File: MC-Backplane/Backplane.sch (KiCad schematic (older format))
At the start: 1 part

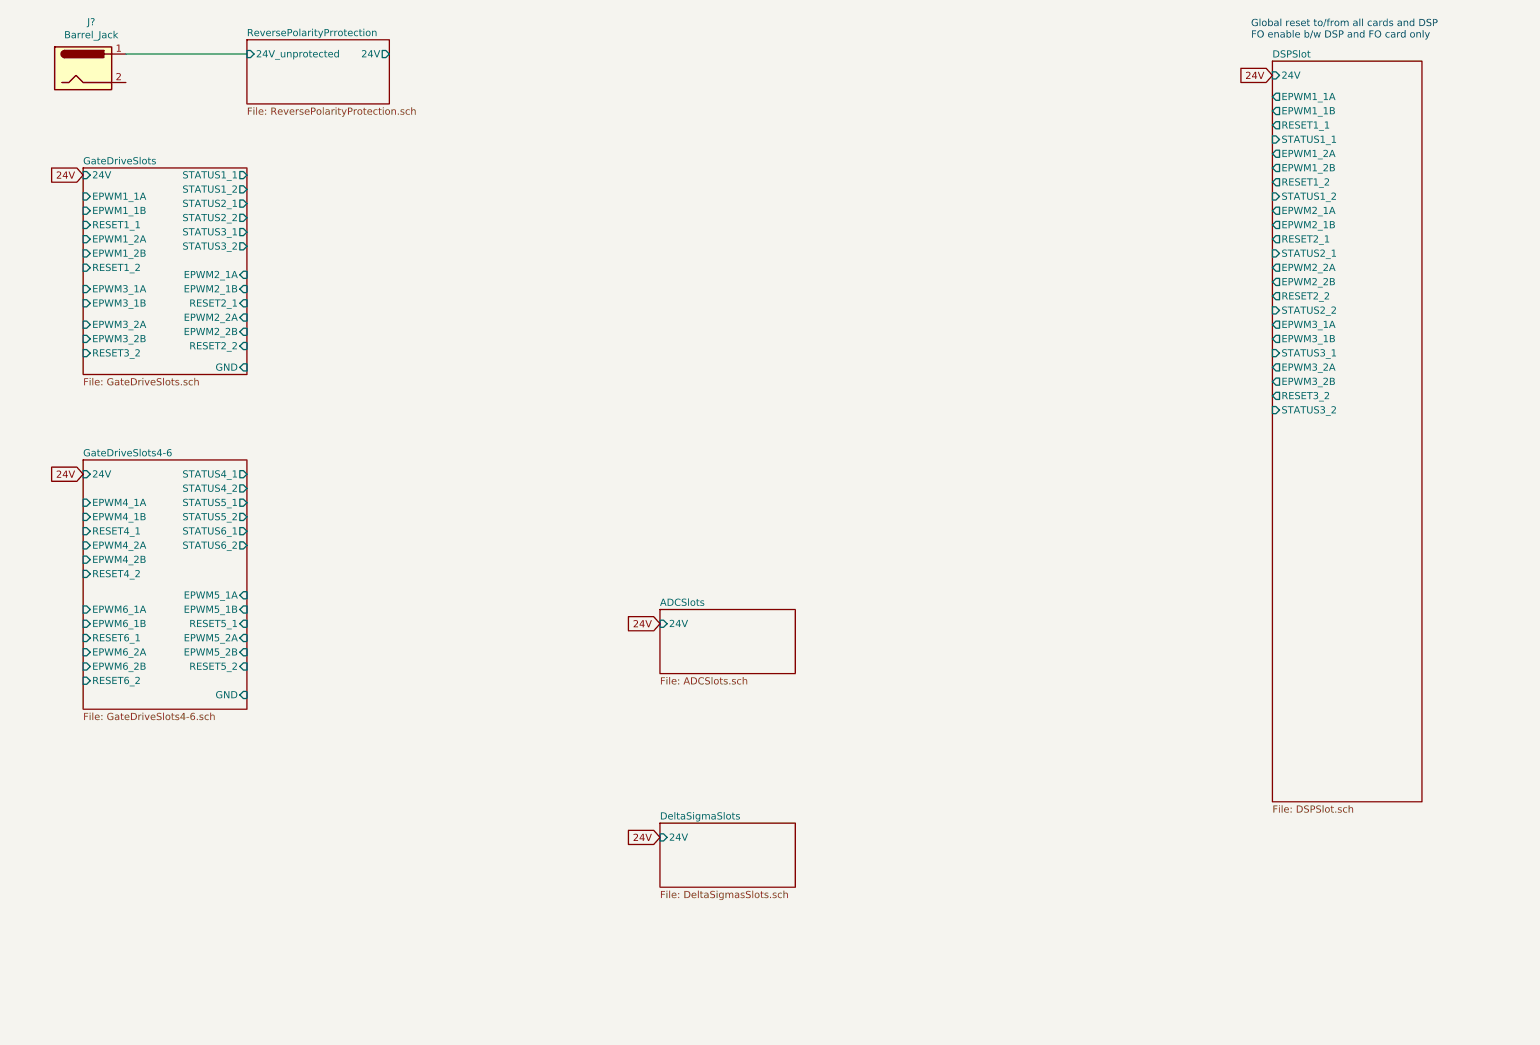
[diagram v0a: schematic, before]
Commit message: Add files via upload
updating net names and wires
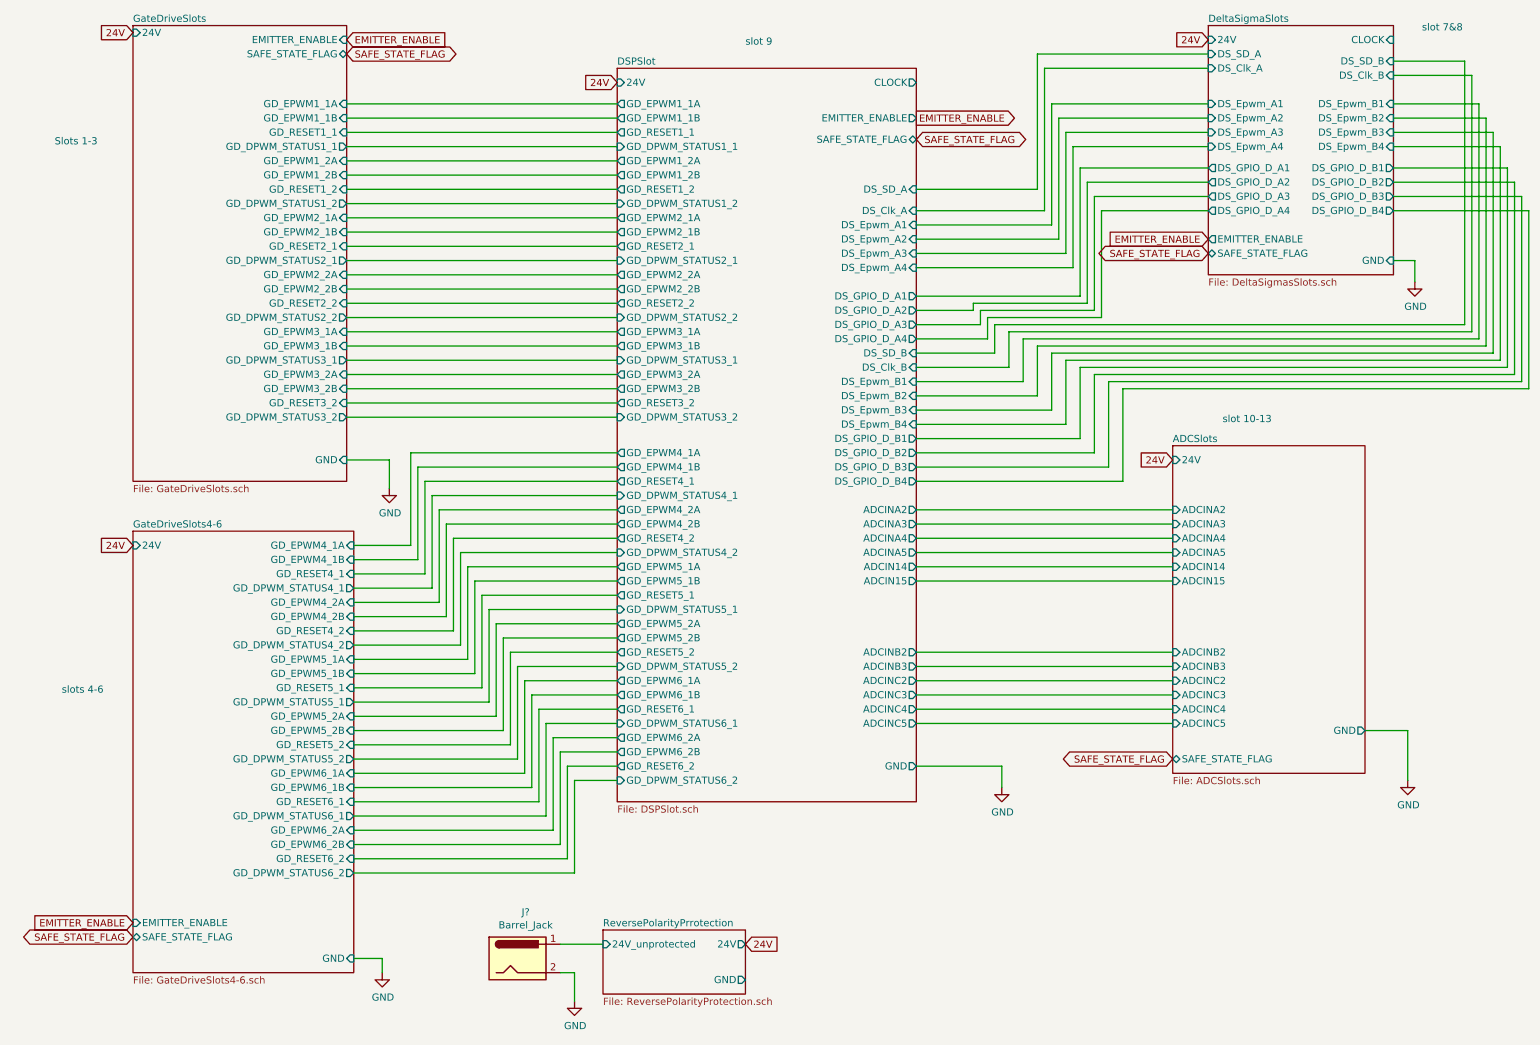
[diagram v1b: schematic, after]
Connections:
- net GND: now reaches J?.2
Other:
- note added: "Slots 1-3"
- note added: "slot 10-13"
- note added: "slot 7&8"
- note added: "slot 9"
- note added: "slots 4-6"
- note removed: "Global reset to/from all cards and DSP\nFO enable b/w DSP and FO card only"
- moved on the sheet: J?
